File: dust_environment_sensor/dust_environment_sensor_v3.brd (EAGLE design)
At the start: 70 x 70 mm, 49 parts, among them IC2 ATMEGA644A, J1 3.6V Lithium C cell, J2 EXP, J3 XBEE_1-10SMT, J4 XBEE_11-20SMT, U1 TSL2560T, U2 LIS3DH, U3 SI7005, U4 TSL2560CL, U5 AMN41121, U6 L3GD20, U7 MCP1700-3.3V, X2 32.768KHz

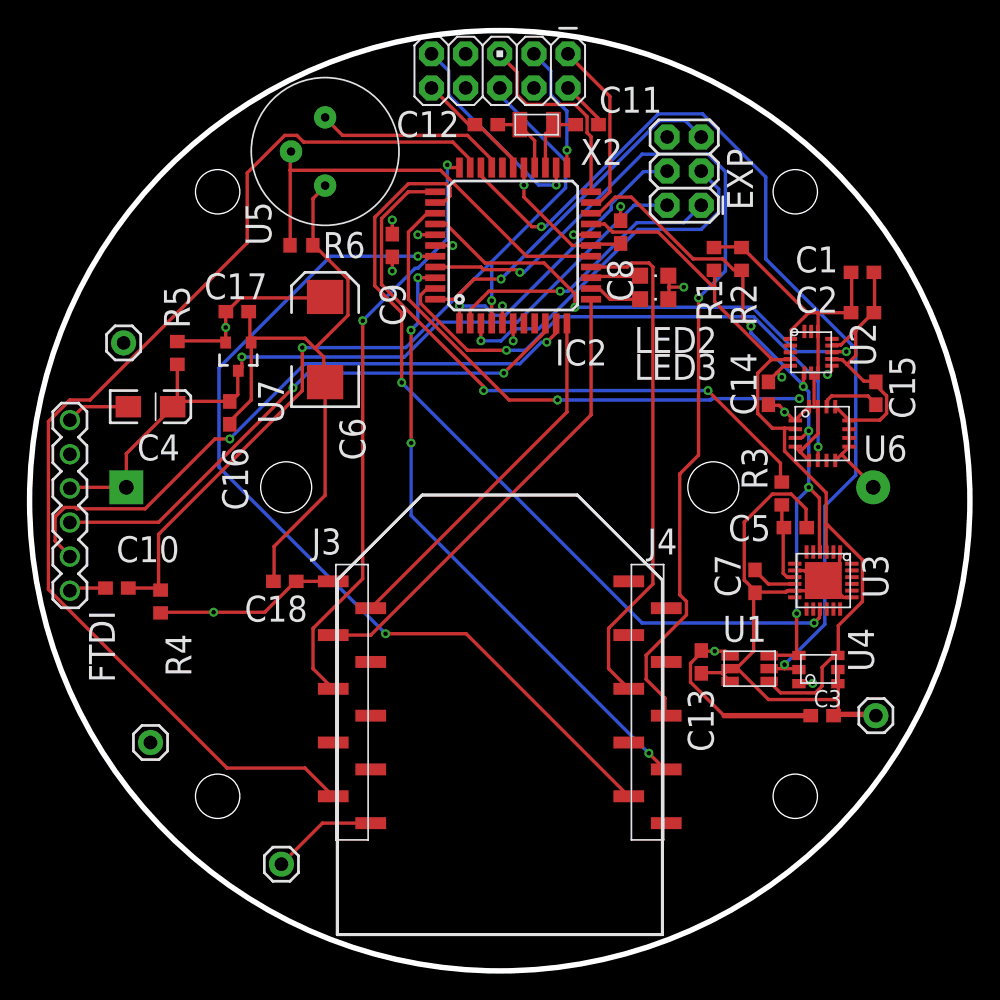
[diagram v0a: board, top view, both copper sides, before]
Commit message: tiny DES3
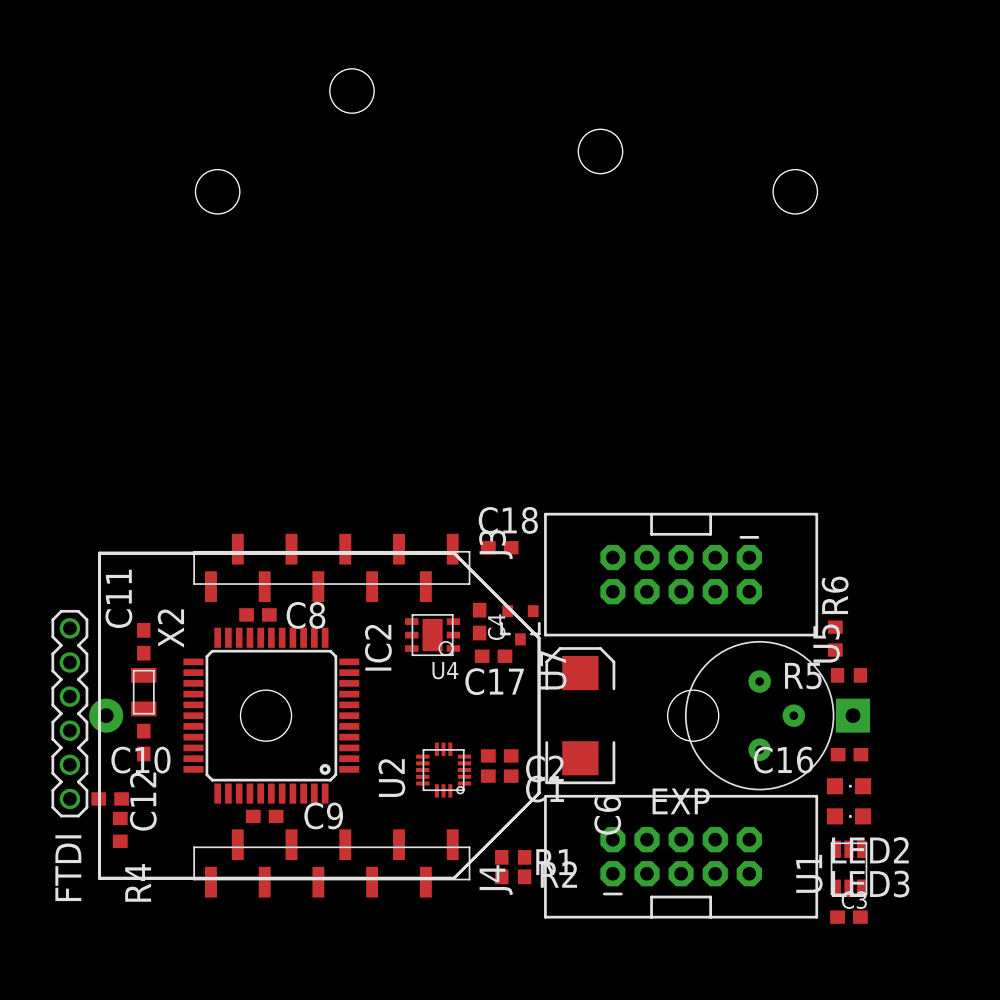
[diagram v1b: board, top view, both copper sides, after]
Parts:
- removed C13, C15, C5: 100n, rcl:C0603
- removed C14: 10u, rcl:C0603
- removed C7: 4.7u, rcl:C0603
- removed J2: EXP, SparkFun-Connectors:2X3
- removed JP4, JP5, JP6, JP7: M01PTH, SparkFun-Connectors:1X01
- removed R3: 15, resistor:R0603
- removed U3: SI7005, Cool_Electricity:QFN24_SILICON_LABS
- removed U6: L3GD20, Cool_Electricity:LGA16_4X4_ST
- added EXP: M05X2SHD, SparkFun-Connectors:2X5-SHROUDED
- C4: value 100u -> 100n; device SparkFun-Capacitors:EIA3216-KIT -> rcl:C0603
- JP9: device SparkFun-Connectors:AVR_ICSP -> SparkFun-Connectors:2X5-SHROUDED
- U4: value TSL2560CL -> HTU21D; device Cool_Electricity:CL6_TAOS -> Cool_Electricity:HTU21D
- moved R5 55.5 mm to (61.0, 22.0), turned to 0 degrees
- moved STANDOFF1 53.4 mm to (24.0, 65.5)
- moved U5 53.0 mm to (54.4, 19.0), turned to 180 degrees
- moved C16 52.7 mm to (61.0, 16.1), turned to 180 degrees
- moved C12 52.6 mm to (8.50, 17.0), turned to 270 degrees
- moved X2 51.4 mm to (8.50, 20.8), turned to 90 degrees
- moved C11 50.7 mm to (8.50, 24.5), turned to 90 degrees
- moved STANDOFF3 50.1 mm to (42.5, 61.0)
- moved R6 49.4 mm to (60.0, 24.7), turned to 270 degrees
- moved R2 49.0 mm to (36.0, 7.00), turned to 180 degrees
- moved R1 47.0 mm to (36.0, 8.45), turned to 180 degrees
- moved C1 46.2 mm to (35.0, 14.5), turned to 180 degrees
- moved C9 43.5 mm to (17.5, 11.5), turned to 180 degrees
- moved C2 42.6 mm to (35.0, 16.0), turned to 180 degrees
- moved U2 41.4 mm to (30.8, 14.9), turned to 180 degrees
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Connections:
- removed net N$1: C7.1, U3.10
- removed net N$11: C5.1, R3.2, U3.9
- removed net N$2: C15.1, U6.14
- new net MOTE_ASSOCIATED: J4.13
- new net MOTE_CONNECT: J3.6
- new net MOTE_SLEEP: J3.4
- new net MOTE_TCPSTATUS: J4.15
- net EXP_CSN: now also EXP.9; no longer J2.5
- net EXP_MISO: now also EXP.5; no longer J2.1
- net EXP_MOSI: now also EXP.8; no longer J2.4
- net EXP_SCK: now also EXP.7; no longer J2.3
- net GND: now also C4.2, EXP.10, EXP.4; no longer C13.2, C14.2, C15.2, C4.C, C5.2, C7.2, J2.6, JP4.1, JP5.1, JP6.1, JP7.1, U3.1, U3.11, U3.19, U3.8, U3.PAD, U4.3, U6.10, U6.11, U6.12, U6.13, U6.8, U6.9
- net GYRO_INT2: no longer U6.6
- net HUMID_CS: no longer U3.15
- net HUMID_VCC: no longer R3.1
- net I2C_SCL: now also EXP.2, U4.6; no longer U3.3, U4.4, U6.2
- net I2C_SDA: now also EXP.1, U4.1; no longer U3.4, U4.5, U6.3
- net LIGHT_INT: no longer U4.6
- net MOTE_ASSOC: no longer J4.15
- net MOTE_STATUS: no longer J4.13
- net VBATT: now also EXP.6; no longer C4.A, J2.2
- net VCC: now also C4.1, EXP.3, U4.5; no longer C13.1, C14.1, U4.1, U6.1, U6.15, U6.16, U6.4, U6.5
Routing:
- net GND: track 165.4 -> 0.00 mm, vias 7 -> 0
- net VCC: track 93.8 -> 0.00 mm, vias 9 -> 0
- net MOTE_SLEEPN: track 84.7 -> 0.00 mm
- net LIGHT_INT: track 72.6 -> 0.00 mm, vias 2 -> 0
- net MOTE_ASSOC: track 70.0 -> 0.00 mm, vias 2 -> 0
- net MOTE_TX_CTSN: track 67.6 -> 0.00 mm, vias 2 -> 0
- net RST: track 63.5 -> 0.00 mm, vias 2 -> 0
- net HUMID_CS: track 61.1 -> 0.00 mm, vias 2 -> 0
- net VBATT: track 59.5 -> 0.00 mm, vias 1 -> 0
- net I2C_SCL: track 58.4 -> 0.00 mm
- net I2C_SDA: track 54.9 -> 0.00 mm, vias 5 -> 0
- net ATMEGA_TO_FTDI: track 47.2 -> 0.00 mm, vias 2 -> 0
- net HUMID_VCC: track 46.6 -> 0.00 mm, vias 2 -> 0
- net MOTE_STATUS: track 46.0 -> 0.00 mm, vias 4 -> 0
- net MOTE_RESETN: track 44.9 -> 0.00 mm, vias 2 -> 0
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- removed copper zone on layer 15, net GND
- removed copper zone on layer 2, net VCC
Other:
- board outline removed
- board text removed: "U4"
